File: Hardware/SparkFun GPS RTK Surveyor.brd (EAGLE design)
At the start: 69.1 x 110.1 mm, 196 parts, among them J13 Internal, J16 microSD, J17 Qwiic Right Angle, J3 USB Female Type C Connector, J4 External, J5 USB Female Type C Connector, J6 Start Base, J7 Power Switch, Q2 MBT3904DW1T1, U10 MCP73833, U2 3.3V, U3 U-BLOX_ZED-F9P, U4 3.3V, U5 ESP-WROOM-32NARROW, U6 CH340C, U7 MAX17048

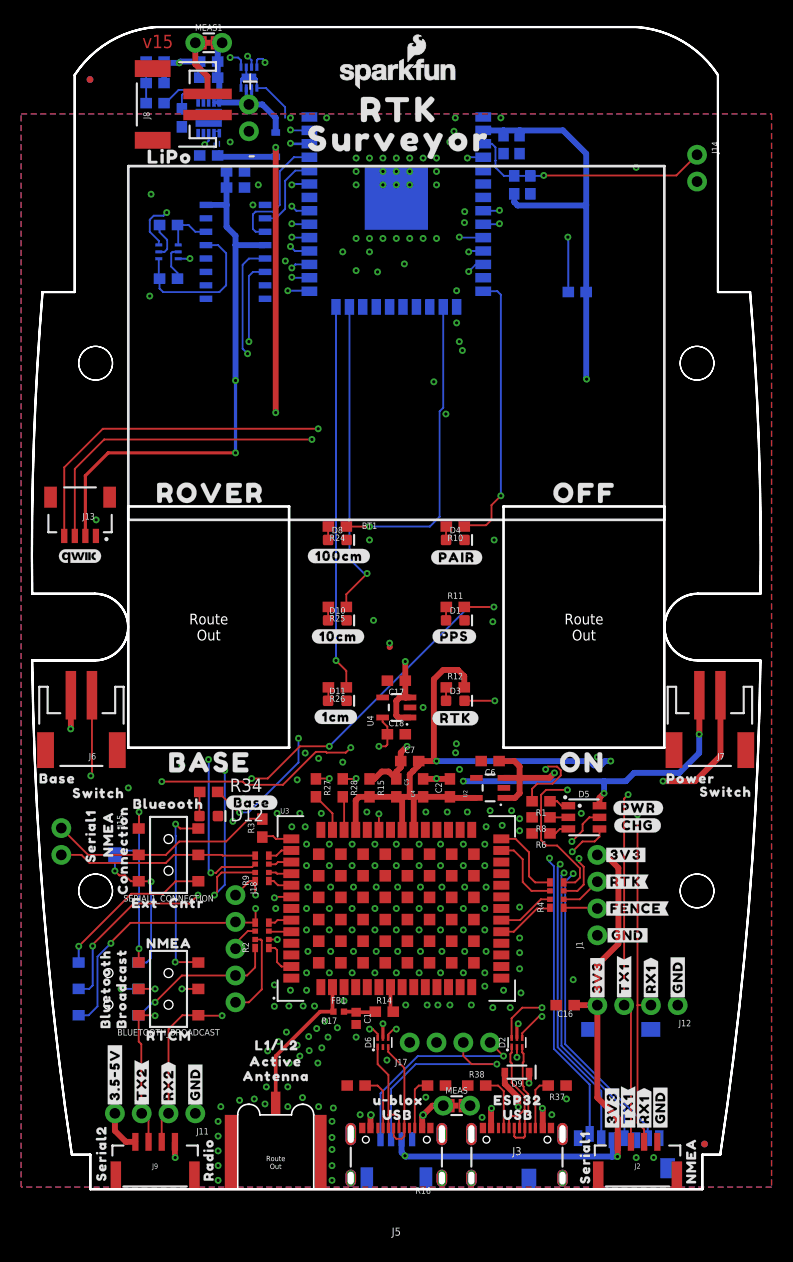
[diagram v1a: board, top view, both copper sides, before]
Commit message: 1x3 panel
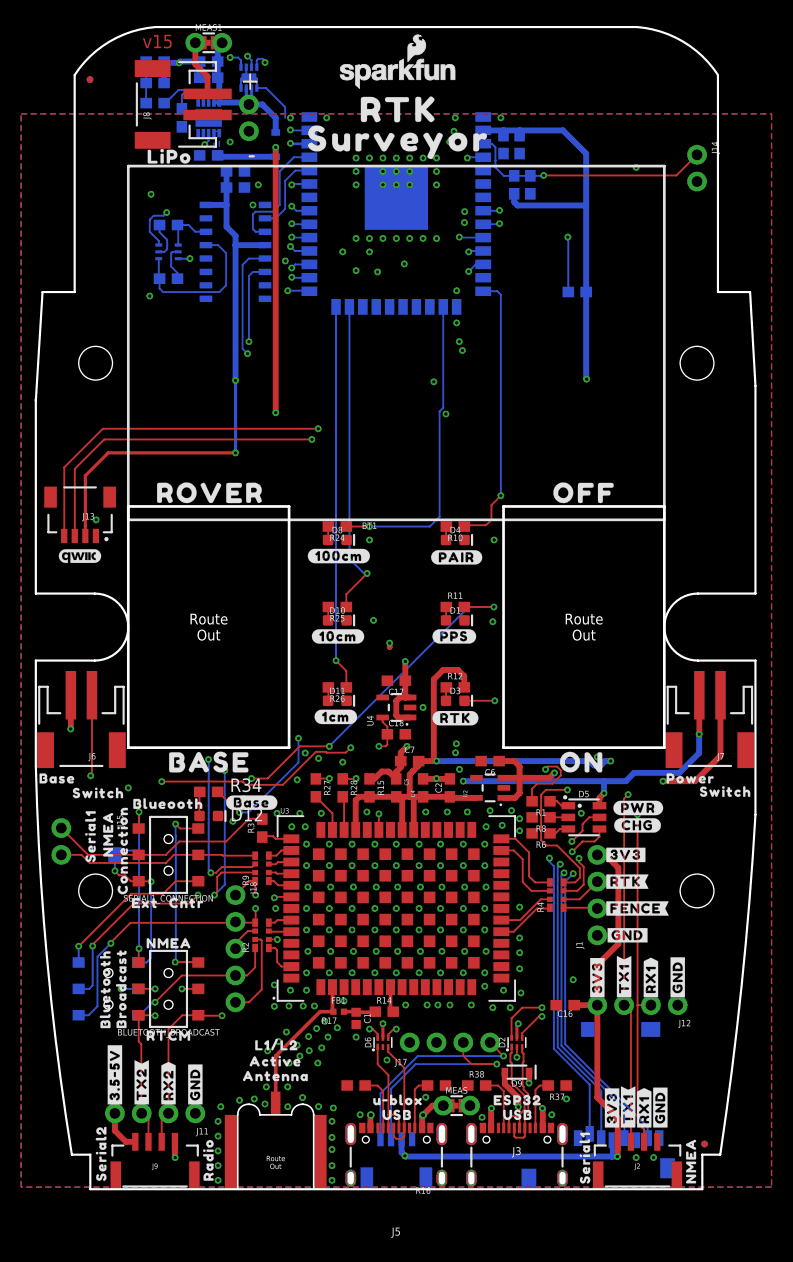
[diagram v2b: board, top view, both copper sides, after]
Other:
- board size 69.1 x 110.1 mm -> 68.2 x 110.1 mm
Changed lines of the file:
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@@
 <layers>
 <layer number="1" name="Top" color="4" fill="1" visible="yes" active="yes"/>
-<layer number="2" name="Horz/GND" color="1" fill="3" visible="yes" active="yes"/>
-<layer number="15" name="Vert" color="4" fill="6" visible="yes" active="yes"/>
+<layer number="2" name="Horz/GND" color="1" fill="3" visible="no" active="yes"/>
+<layer number="15" name="Vert" color="4" fill="6" visible="no" active="yes"/>
 <layer number="16" name="Bottom" color="1" fill="1" visible="yes" active="yes"/>
 <layer number="17" name="Pads" color="2" fill="1" visible="yes" active="yes"/>
@@
 <layer number="23" name="tOrigins" color="15" fill="1" visible="yes" active="yes"/>
 <layer number="24" name="bOrigins" color="15" fill="1" visible="yes" active="yes"/>
-<layer number="25" name="tNames" color="7" fill="1" visible="yes" active="yes"/>
-<layer number="26" name="bNames" color="7" fill="1" visible="yes" active="yes"/>
-<layer number="27" name="tValues" color="7" fill="1" visible="yes" active="yes"/>
-<layer number="28" name="bValues" color="7" fill="1" visible="yes" active="yes"/>
-<layer number="29" name="tStop" color="7" fill="3" visible="yes" active="yes"/>
-<layer number="30" name="bStop" color="7" fill="6" visible="yes" active="yes"/>
-<layer number="31" name="tCream" color="7" fill="4" visible="yes" active="yes"/>
-<layer number="32" name="bCream" color="7" fill="5" visible="yes" active="yes"/>
-<layer number="33" name="tFinish" color="6" fill="3" visible="yes" active="yes"/>
-<layer number="34" name="bFinish" color="6" fill="6" visible="yes" active="yes"/>
-<layer number="35" name="tGlue" color="7" fill="4" visible="yes" active="yes"/>
-<layer number="36" name="bGlue" color="7" fill="5" visible="yes" active="yes"/>
-<layer number="37" name="tTest" color="7" fill="1" visible="yes" active="yes"/>
-<layer number="38" name="bTest" color="7" fill="1" visible="yes" active="yes"/>
-<layer number="39" name="tKeepout" color="4" fill="11" visible="yes" active="yes"/>
-<layer number="40" name="bKeepout" color="1" fill="11" visible="yes" active="yes"/>
-<layer number="41" name="tRestrict" color="4" fill="10" visible="yes" active="yes"/>
-<layer number="42" name="bRestrict" color="1" fill="10" visible="yes" active="yes"/>
-<layer number="43" name="vRestrict" color="2" fill="10" visible="yes" active="yes"/>
-<layer number="44" name="Drills" color="7" fill="1" visible="yes" active="yes"/>
+<layer number="25" name="tNames" color="7" fill="1" visible="no" active="yes"/>
+<layer number="26" name="bNames" color="7" fill="1" visible="no" active="yes"/>
+<layer number="27" name="tValues" color="7" fill="1" visible="no" active="yes"/>
+<layer number="28" name="bValues" color="7" fill="1" visible="no" active="yes"/>
+<layer number="29" name="tStop" color="7" fill="3" visible="no" active="yes"/>
+<layer number="30" name="bStop" color="7" fill="6" visible="no" active="yes"/>
+<layer number="31" name="tCream" color="7" fill="4" visible="no" active="yes"/>
+<layer number="32" name="bCream" color="7" fill="5" visible="no" active="yes"/>
+<layer number="33" name="tFinish" color="6" fill="3" visible="no" active="yes"/>
+<layer number="34" name="bFinish" color="6" fill="6" visible="no" active="yes"/>
+<layer number="35" name="tGlue" color="7" fill="4" visible="no" active="yes"/>
+<layer number="36" name="bGlue" color="7" fill="5" visible="no" active="yes"/>
+<layer number="37" name="tTest" color="7" fill="1" visible="no" active="yes"/>
+<layer number="38" name="bTest" color="7" fill="1" visible="no" active="yes"/>
+<layer number="39" name="tKeepout" color="4" fill="11" visible="no" active="yes"/>
+<layer number="40" name="bKeepout" color="1" fill="11" visible="no" active="yes"/>
+<layer number="41" name="tRestrict" color="4" fill="10" visible="no" active="yes"/>
+<layer number="42" name="bRestrict" color="1" fill="10" visible="no" active="yes"/>
+<layer number="43" name="vRestrict" color="2" fill="10" visible="no" active="yes"/>
+<layer number="44" name="Drills" color="7" fill="1" visible="no" active="yes"/>
 <layer number="45" name="Holes" color="7" fill="1" visible="yes" active="yes"/>
-<layer number="46" name="Milling" color="3" fill="1" visible="yes" active="yes"/>
-<layer number="47" name="Measures" color="7" fill="1" visible="yes" active="yes"/>
-<layer number="48" name="Document" color="7" fill="1" visible="yes" active="yes"/>
+<layer number="46" name="Milling" color="3" fill="1" visible="no" active="yes"/>
+<layer number="47" name="Measures" color="7" fill="1" visible="no" active="yes"/>
+<layer number="48" name="Document" color="7" fill="1" visible="no" active="yes"/>
 <layer number="49" name="Reference" color="7" fill="1" visible="yes" active="yes"/>
-<layer number="50" name="dxf" color="7" fill="1" visible="yes" active="yes"/>
+<layer number="50" name="dxf" color="7" fill="1" visible="no" active="yes"/>
 <layer number="51" name="tDocu" color="6" fill="1" visible="yes" active="yes"/>
-<layer number="52" name="bDocu" color="7" fill="1" visible="yes" active="yes"/>
+<layer number="52" name="bDocu" color="7" fill="1" visible="no" active="yes"/>
 <layer number="91" name="Nets" color="2" fill="1" visible="no" active="no"/>
 <layer number="92" name="Busses" color="1" fill="1" visible="no" active="no"/>
@@
 <text x="25.4" y="2" size="0.5" layer="51" ratio="20" rot="R180" align="center">Connectors</text>
 <wire x1="2.5908" y1="110.205" x2="48.2092" y2="110.205" width="0.2032" layer="20"/>
-<hole x="-3.0988" y="28.3337" drill="3.2004"/>
-<hole x="-3.0988" y="78.3463" drill="3.2004"/>
-<hole x="53.8988" y="78.3463" drill="3.2004"/>
-<hole x="53.8988" y="28.3337" drill="3.2004"/>
-<wire x1="-9.1092" y1="50.1777" x2="-3.175" y2="50.1777" width="0.2032" layer="20"/>
-<wire x1="-3.175" y1="56.5023" x2="-9.1092" y2="56.5023" width="0.2032" layer="20"/>
 <wire x1="-6.3119" y1="102.87" x2="2.5908" y2="110.205" width="0.2032" layer="51" curve="-72.045824"/>
-<wire x1="-9.1092" y1="56.5023" x2="-6.3119" y2="102.87" width="0.2032" layer="51" curve="-8.331372"/>
-<wire x1="-3.175" y1="50.1777" x2="-3.175" y2="56.5023" width="0.2032" layer="20" curve="180"/>
-<wire x1="59.9092" y1="50.1777" x2="53.975" y2="50.1777" width="0.2032" layer="20"/>
-<wire x1="53.975" y1="56.5023" x2="59.9092" y2="56.5023" width="0.2032" layer="20"/>
-<wire x1="53.975" y1="50.1777" x2="53.975" y2="56.5023" width="0.2032" layer="20" curve="-180"/>
-<wire x1="-8.128" y1="85.09" x2="-5.08" y2="85.09" width="0.2032" layer="20"/>
-<wire x1="-5.08" y1="85.09" x2="-5.08" y2="105.664" width="0.2032" layer="20"/>
-<wire x1="-9.1092" y1="56.5023" x2="-8.128" y2="85.09" width="0.2032" layer="20" curve="-5.381392"/>
-<wire x1="-5.08" y1="105.664" x2="2.5908" y2="110.205" width="0.2032" layer="20" curve="-52.405474"/>
+<wire x1="-3.175" y1="50.165" x2="-3.175" y2="56.515" width="0.2032" layer="20" curve="180"/>
+<wire x1="53.975" y1="50.165" x2="53.975" y2="56.515" width="0.2032" layer="20" curve="-180"/>
 <wire x1="-3.6" y1="0.065" x2="54.4" y2="0.065" width="0.2032" layer="20"/>
 <wire x1="-3.6" y1="0.065" x2="-3.6" y2="3.34" width="0.2032" layer="20"/>
@@
 <wire x1="54.4" y1="0.065" x2="54.4" y2="3.34" width="0.2032" layer="20"/>
 <wire x1="54.4" y1="3.34" x2="56.1" y2="3.34" width="0.2032" layer="20"/>
-<wire x1="-5.35" y1="3.34" x2="-9.1092" y2="50.1777" width="0.2032" layer="20" curve="-7.756885"/>
-<wire x1="56.1" y1="3.34" x2="59.9092" y2="50.1777" width="0.2032" layer="20" curve="7.756885"/>
+<wire x1="-5.35" y1="3.34" x2="-8.763" y2="40.132" width="0.2032" layer="20" curve="-7.756885"/>
+<wire x1="56.1" y1="3.34" x2="59.436" y2="35.56" width="0.2032" layer="20" curve="5.151818"/>
 <wire x1="57.1119" y1="102.87" x2="48.2092" y2="110.205" width="0.2032" layer="51" curve="72.045824"/>
-<wire x1="59.9092" y1="56.5023" x2="57.1119" y2="102.87" width="0.2032" layer="51" curve="8.331372"/>
+<wire x1="-8.763" y1="40.132" x2="-8.763" y2="50.165" width="0.2032" layer="20"/>
+<wire x1="-8.763" y1="50.165" x2="-3.175" y2="50.165" width="0.2032" layer="20"/>
+<wire x1="-8.763" y1="56.515" x2="-8.763" y2="74.803" width="0.2032" layer="20"/>
+<wire x1="-8.763" y1="74.803" x2="-8.763" y2="74.93" width="0.2032" layer="20"/>
+<wire x1="-8.763" y1="56.515" x2="-3.175" y2="56.515" width="0.2032" layer="20"/>
+<wire x1="59.436" y1="50.165" x2="59.436" y2="35.56" width="0.2032" layer="20"/>
+<wire x1="59.436" y1="50.165" x2="53.975" y2="50.165" width="0.2032" layer="20"/>
+<wire x1="59.436" y1="56.515" x2="59.436" y2="76.2" width="0.2032" layer="20"/>
+<wire x1="59.436" y1="56.515" x2="53.975" y2="56.515" width="0.2032" layer="20"/>
+<wire x1="57.1119" y1="102.87" x2="48.2092" y2="110.205" width="0.2032" layer="51" curve="72.045824"/>
 <wire x1="58.928" y1="85.09" x2="55.88" y2="85.09" width="0.2032" layer="20"/>
 <wire x1="55.88" y1="85.09" x2="55.88" y2="105.664" width="0.2032" layer="20"/>
-<wire x1="59.9092" y1="56.5023" x2="58.928" y2="85.09" width="0.2032" layer="20" curve="5.381392"/>
 <wire x1="55.88" y1="105.664" x2="48.2092" y2="110.205" width="0.2032" layer="20" curve="52.405474"/>
+<wire x1="-8.128" y1="85.09" x2="-5.08" y2="85.09" width="0.2032" layer="20"/>
+<wire x1="-5.08" y1="85.09" x2="-5.08" y2="105.664" width="0.2032" layer="20"/>
+<wire x1="-5.08" y1="105.664" x2="2.5908" y2="110.205" width="0.2032" layer="20" curve="-52.405474"/>
+<wire x1="-8.763" y1="74.803" x2="-8.128" y2="85.09" width="0.2032" layer="20"/>
+<wire x1="59.436" y1="76.2" x2="58.928" y2="85.09" width="0.2032" layer="20"/>
 </plain>
 <attributes>
